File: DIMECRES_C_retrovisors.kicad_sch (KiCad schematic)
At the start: 84 parts, among them J10 Vbat, J2 DE9_Pins, J3 Conn_01x05_Pin, J4 Motor3, J5 DE9_Pins, J6 Intermitente, J7 Calentador, J8 Motor2, J9 Motor1, Q1 DTC144E, Q2 DTC144E, Q3 DTC144E, SW1 SW_DPDT_G6S, SW10 SW_Push, SW2 SW_Push, SW3 SW_Push, SW4 SW_Push, SW5 SW_Push, SW6 SW_Push, SW7 SW_Push, SW8 FN01B, SW9 FN01B, U1 CH201, U10 LM1117DT-5.0, U2 ADM7160, U3 LM2596S-ADJ, U4 L298N, U5 MCP2551-I-SN, U6 ADA4511-2, U7 PIC18F4480-IP, Y1 Crystal

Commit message: lop
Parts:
- R22, R23, R24: footprint (none) -> Resistor_SMD:R_0805_2012Metric_Pad1.20x1.40mm_HandSolder
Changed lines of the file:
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@@
 			)
 		)
-		(property "Footprint" ""
+		(property "Footprint" "Resistor_SMD:R_0805_2012Metric_Pad1.20x1.40mm_HandSolder"
 			(at 214.122 269.24 90)
 			(effects
@@
 			)
 		)
-		(property "Footprint" ""
+		(property "Footprint" "Resistor_SMD:R_0805_2012Metric_Pad1.20x1.40mm_HandSolder"
 			(at 335.407 245.745 90)
 			(effects
@@
 			)
 		)
-		(property "Footprint" ""
+		(property "Footprint" "Resistor_SMD:R_0805_2012Metric_Pad1.20x1.40mm_HandSolder"
 			(at 356.362 102.87 90)
 			(effects

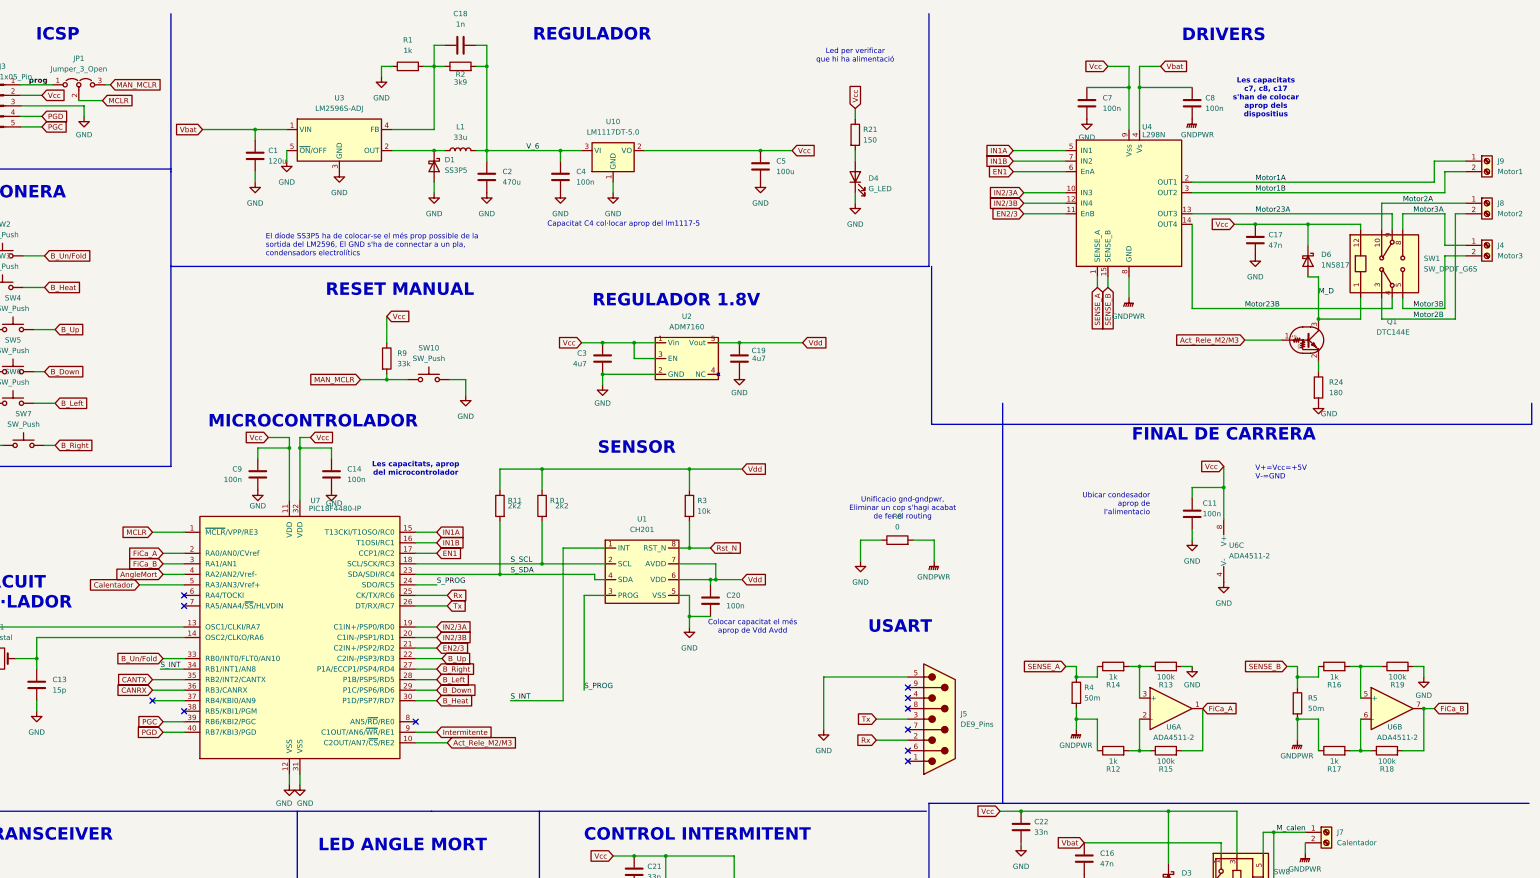
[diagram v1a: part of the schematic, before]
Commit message: Proimeres correccions
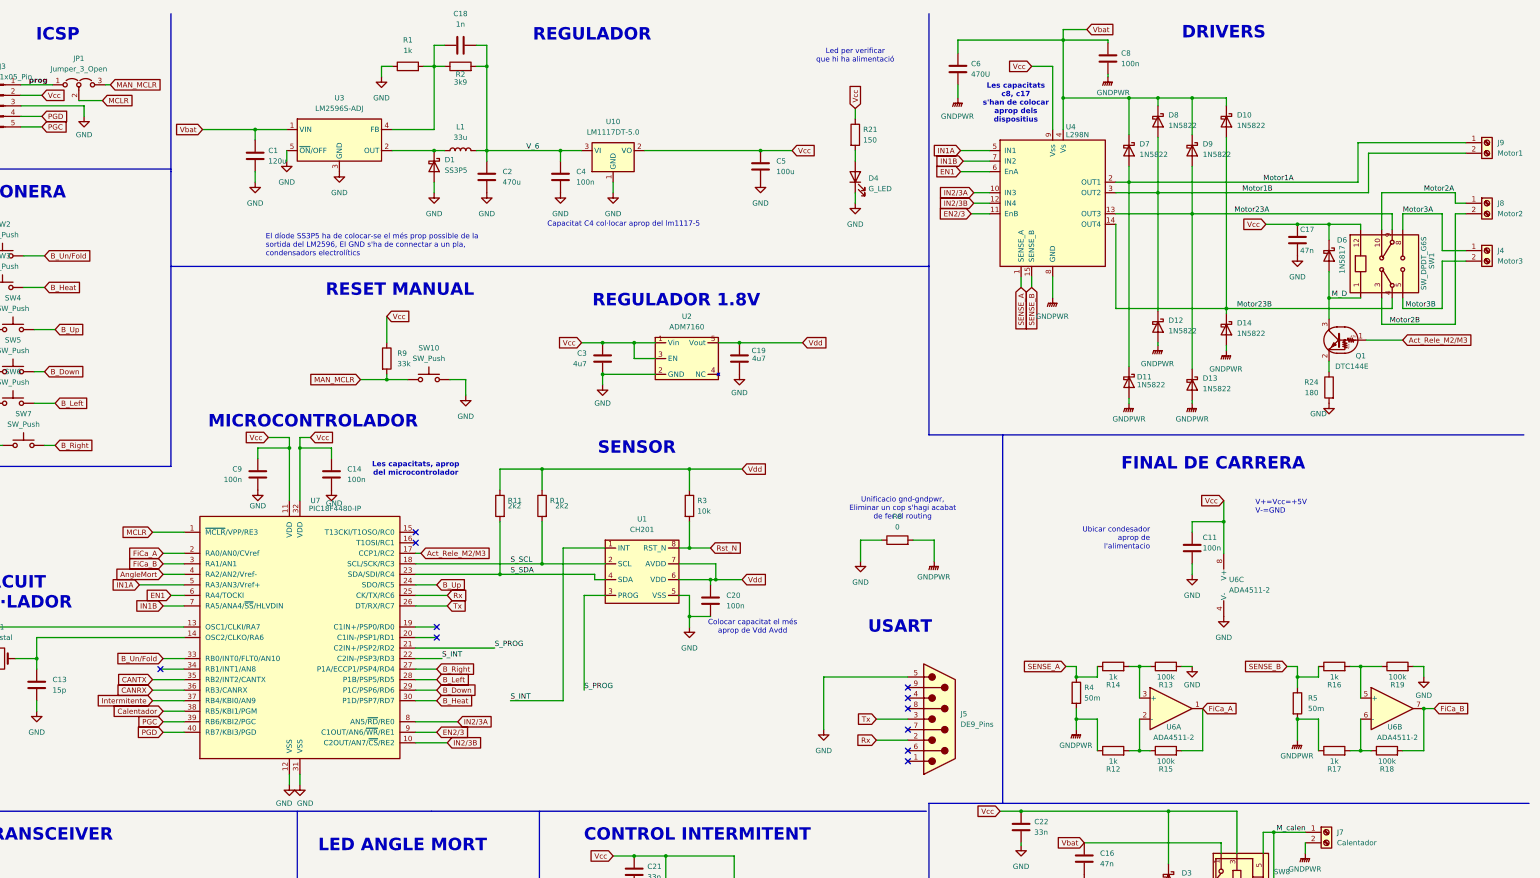
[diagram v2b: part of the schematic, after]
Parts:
- removed C7: 100n, Capacitor_SMD:C_1206_3216Metric_Pad1.33x1.80mm_HandSolder, symbol Device:C
- added C6: 470U, Capacitor_THT:CP_Radial_D6.3mm_P2.50mm, symbol Device:C
- added D10, D11, D12, D13, D14, D7, D8, D9: 1N5822, Diode_THT:D_DO-201AD_P15.24mm_Horizontal, symbol Diode:1N5822
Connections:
- net Act_Rele_M2/M3: now also U7.17 (CCP1/RC2); no longer U7.10 (C2OUT/AN7/~{CS}/RE2)
- net B_Up: now also U7.24 (SDO/RC5); no longer U7.22 (C2IN-/PSP3/RD3)
- net Calentador: now also U7.38 (RB5/KBI1/PGM); no longer U7.5 (RA3/AN3/Vref+)
- net EN1: now also U7.6 (RA4/TOCKI); no longer U7.17 (CCP1/RC2)
- net EN2/3: now also U7.9 (C1OUT/AN6/~{WR}/RE1); no longer U7.21 (C2IN+/PSP2/RD2)
- net GNDPWR: now also C6.2, D11.2 (A), D12.2 (A), D13.2 (A), D14.2 (A)
- net IN1A: now also U7.5 (RA3/AN3/Vref+); no longer U7.15 (T13CKI/T1OSO/RC0)
- net IN1B: now also U7.7 (RA5/ANA4/~{SS}/HLVDIN); no longer U7.16 (T1OSI/RC1)
- net IN2/3A: now also U7.8 (AN5/~{RD}/RE0); no longer U7.19 (C1IN+/PSP0/RD0)
- net IN2/3B: now also U7.10 (C2OUT/AN7/~{CS}/RE2); no longer U7.20 (C1IN-/PSP1/RD1)
- net Intermitente: now also U7.37 (RB4/KBI0/AN9); no longer U7.9 (C1OUT/AN6/~{WR}/RE1)
- net Motor1A: now also D11.1 (K), D7.2 (A)
- net Motor1B: now also D12.1 (K), D8.2 (A)
- net Motor23A: now also D13.1 (K), D9.2 (A)
- net Motor23B: now also D10.2 (A), D14.1 (K)
- net S_INT: now also U7.22 (C2IN-/PSP3/RD3); no longer U7.34 (RB1/INT1/AN8)
- net S_PROG: now also U7.21 (C2IN+/PSP2/RD2); no longer U7.24 (SDO/RC5)
- net Vbat: now also C6.1, D10.1 (K), D7.1 (K), D8.1 (K), D9.1 (K)
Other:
- note added: "Les capacitats c8, c17 s'han de colocar aprop dels dispositius"
- note removed: "Les capacitats c7, c8, c17 s'han de colocar aprop dels dispositius"
- moved on the sheet: C11, C17, C8, D6, J4, J9, Q1, R24, U4, U6C
